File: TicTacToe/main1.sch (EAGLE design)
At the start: 33 parts, among them U1 ATMEGA168-20AU, X2 MINI-USB-SHIELD-UX60A-MB-5ST

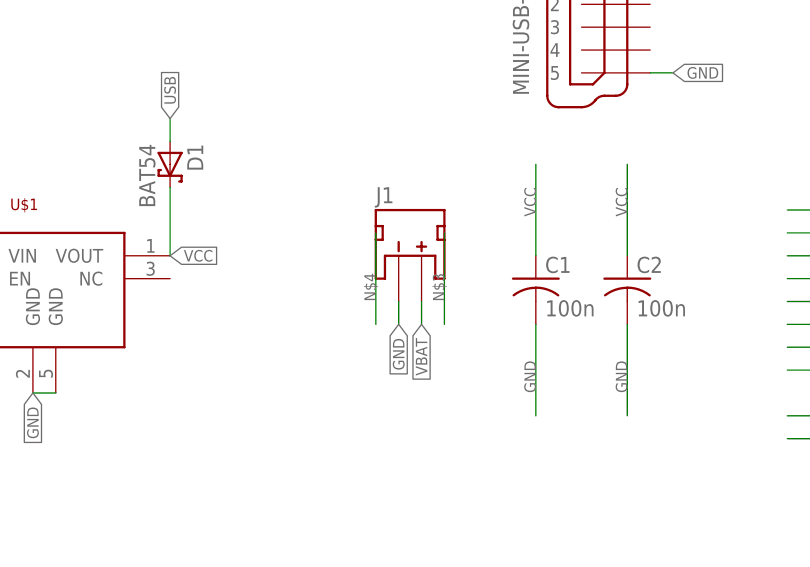
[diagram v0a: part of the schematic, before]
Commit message: updated project
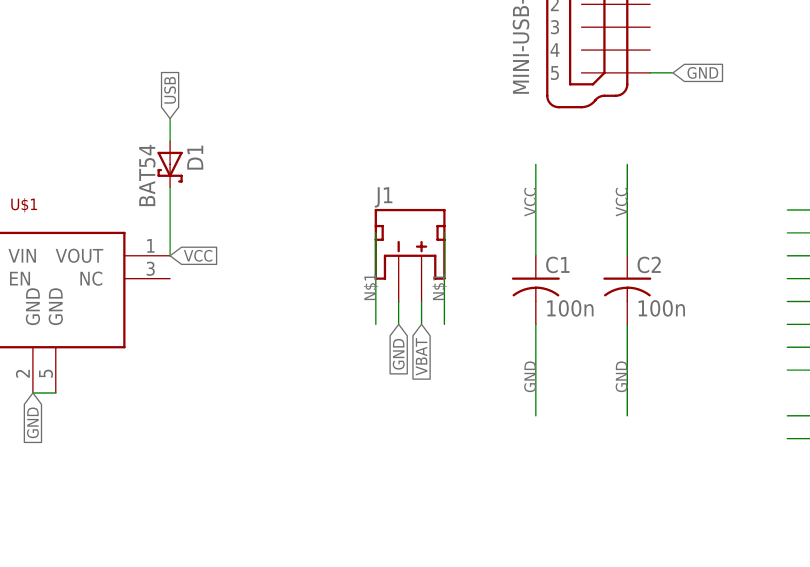
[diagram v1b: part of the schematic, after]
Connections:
- removed net N$3: J1.PAD2
- removed net N$4: J1.PAD1
- new net N$1: J1.PAD1, J1.PAD2
